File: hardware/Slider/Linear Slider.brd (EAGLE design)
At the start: 89.4 x 17.5 mm, 9 parts

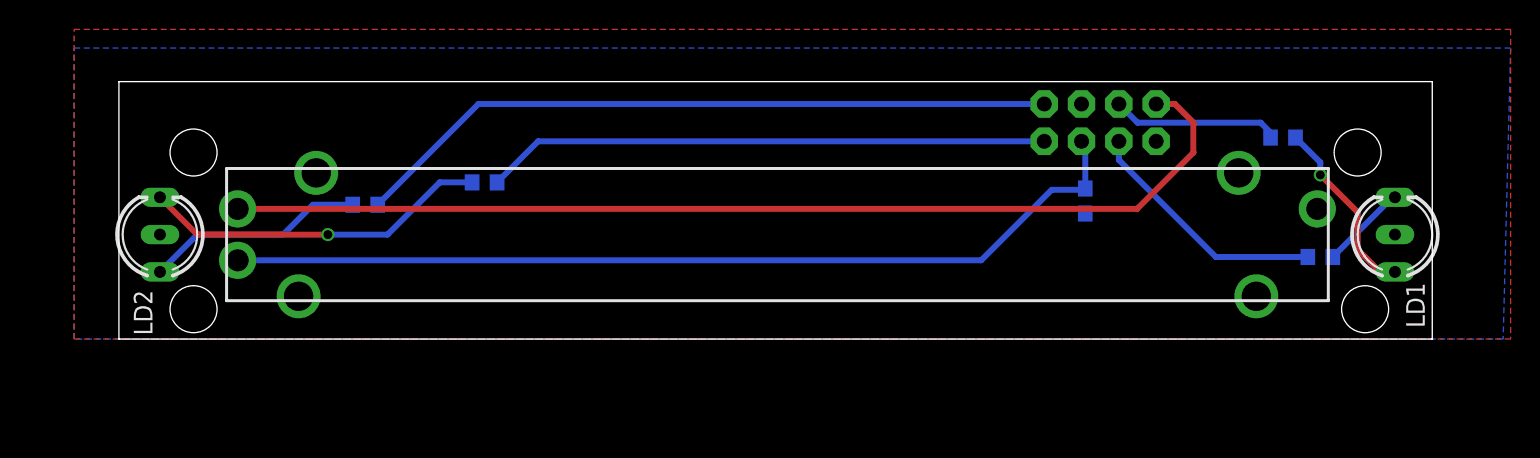
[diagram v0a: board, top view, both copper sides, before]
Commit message: Updates
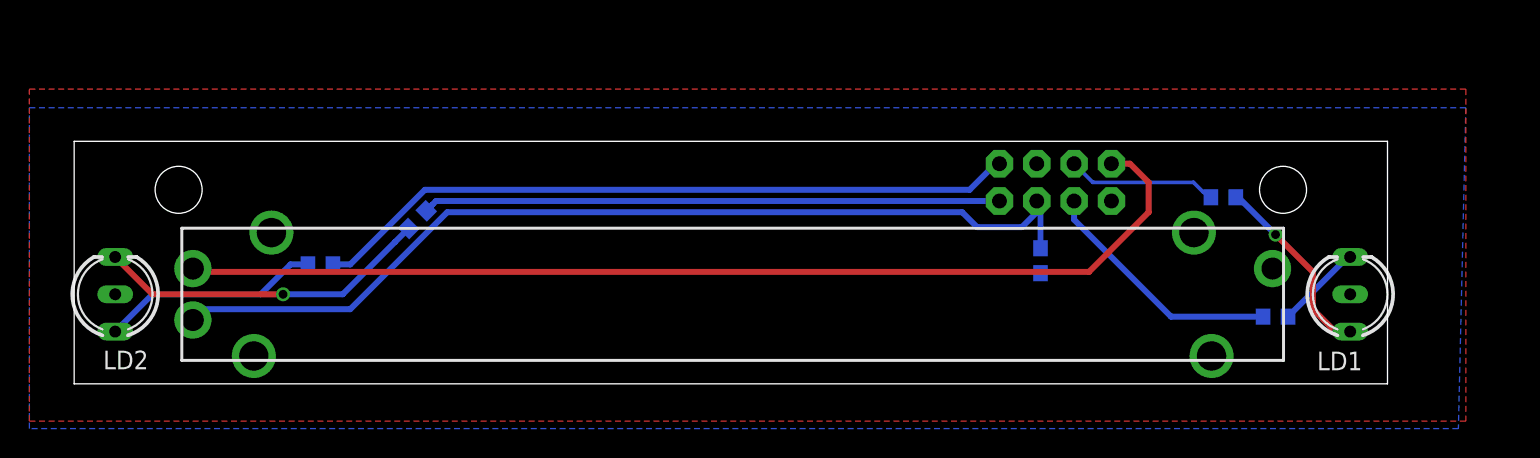
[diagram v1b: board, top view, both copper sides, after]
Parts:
- moved R2 5.75 mm to (78.2, 12.7)
- moved R3 5.23 mm to (23.4, 11.2), turned to 135 degrees
- moved C1 5.08 mm to (65.8, 8.38)
- moved LD1 5.08 mm to (86.9, 6.10)
- moved R1 5.08 mm to (81.8, 4.57)
- moved R4 5.08 mm to (16.8, 8.13)
- moved LD2 5.08 mm to (2.79, 6.10)
- moved POT1 5.08 mm to (44.8, 6.10)
- moved SERIAL 5.08 mm to (66.8, 13.7)
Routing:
- net SLIDER_IN: track 63.0 -> 65.5 mm
- net LED_TOP_G: track 11.5 -> 10.2 mm
- net N$4: track 23.8 -> 22.9 mm
- net LED_BOT_R: track 38.4 -> 39.3 mm
- net N$2: track 12.5 -> 13.1 mm
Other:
- board size 89.4 x 17.5 mm -> 89.4 x 16.5 mm
- board text added: "peschuster.de - 05/2013"
